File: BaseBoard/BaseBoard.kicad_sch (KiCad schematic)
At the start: 33 parts, among them J1 IMU, J13 Conn_01x02_Female, J14 Conn_01x03_Female, J2 Conn_01x04, J3 Raspberry_Pi_2_3, J4 USB_C_Receptacle_USB2.0, J5 Conn_02x04, SW1 SW_Push, SW2 SW_Push, U1 GD32VF103C8Tx, Y1 8Mhz

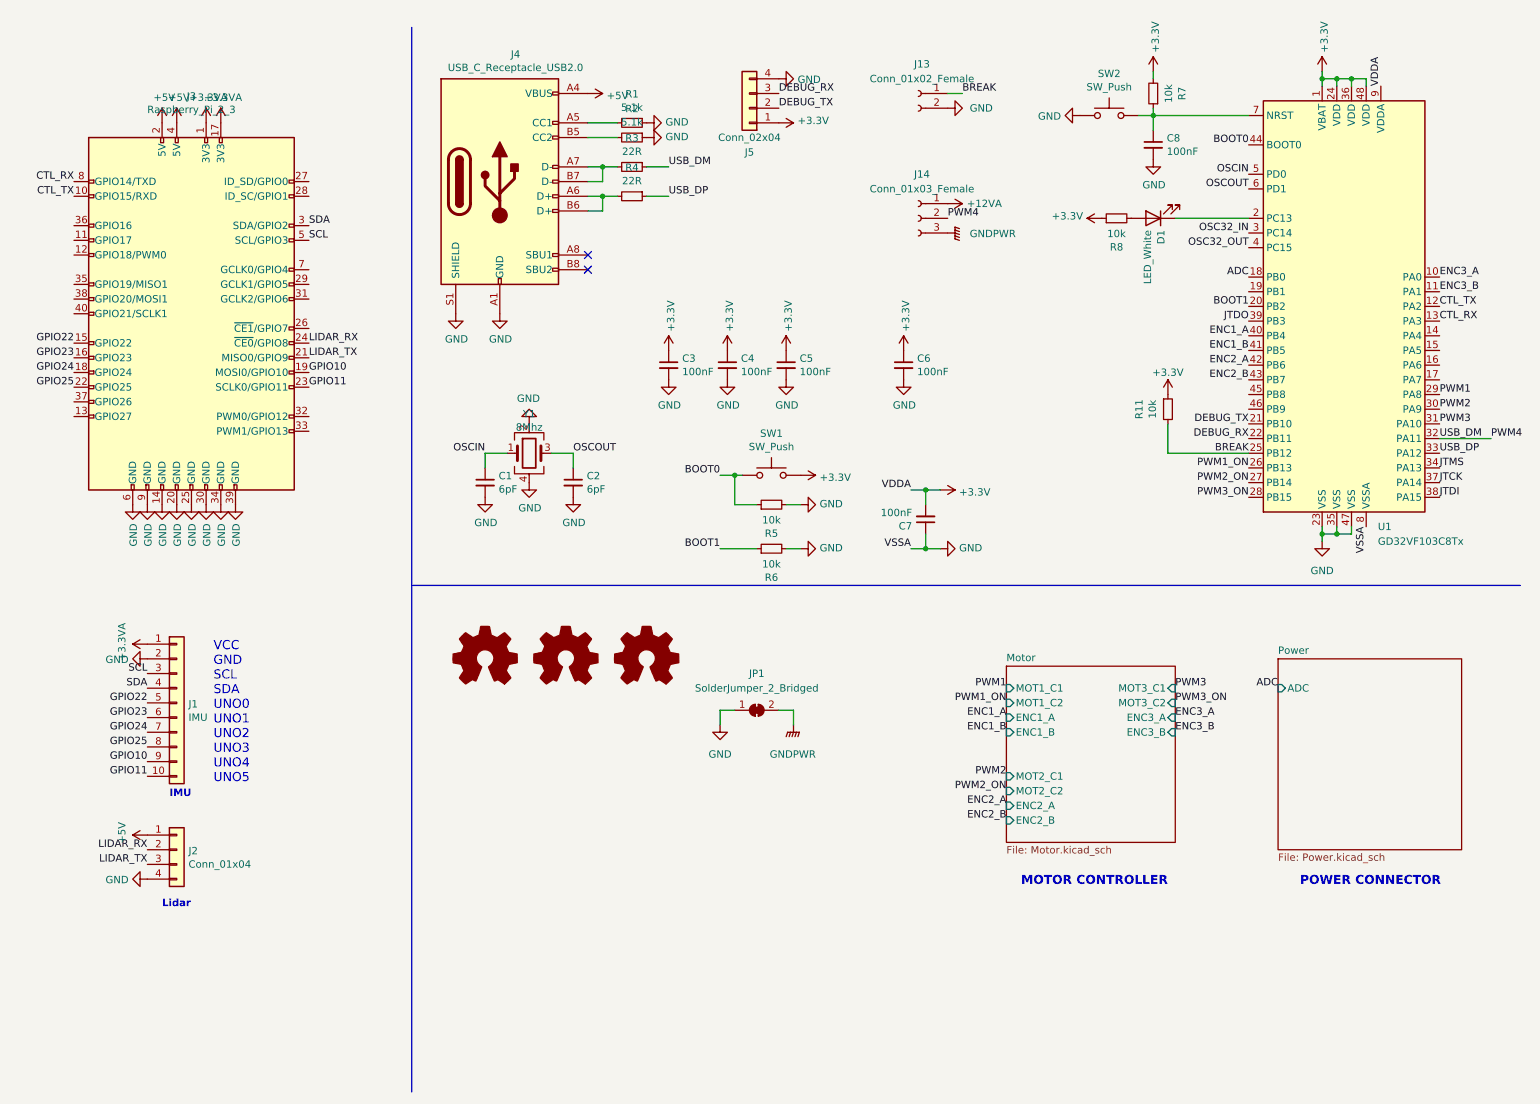
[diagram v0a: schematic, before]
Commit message: 更新V3线路板
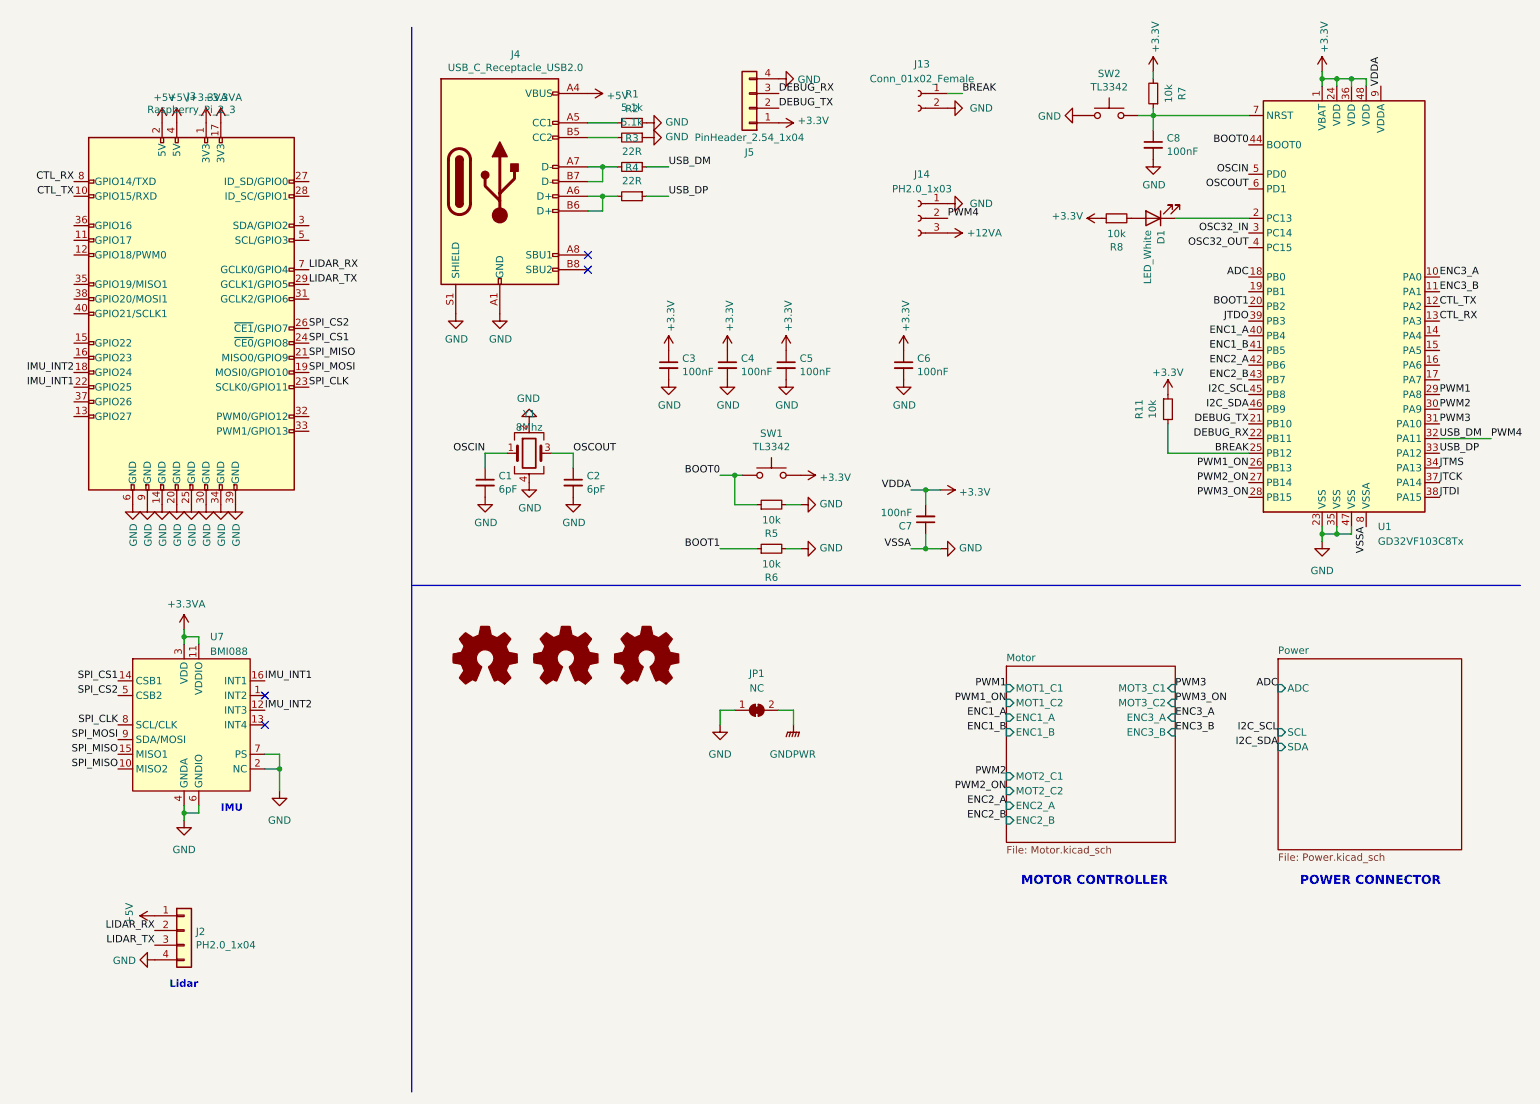
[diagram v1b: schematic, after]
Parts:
- removed J1: IMU, Connector_PinSocket_2.54mm:PinSocket_1x10_P2.54mm_Vertical, symbol Connector_Generic:Conn_01x10
- added U7: BMI088, Smallbot:Bochs_LGA16_2x7+2x1, symbol Smallbot:BMI088
- J14: value Conn_01x03_Female -> PH2.0_1x03
- J2: value Conn_01x04 -> PH2.0_1x04
- J5: value Conn_02x04 -> PinHeader_2.54_1x04
- JP1: value SolderJumper_2_Bridged -> NC
- SW1, SW2: value SW_Push -> TL3342; footprint User_Button_Switch:SW_SPST_EVQP7C-Single -> Button_Switch_SMD:SW_SPST_TL3342
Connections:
- net +12VA: now also J14.3 (Pin_3); no longer J14.1 (Pin_1)
- net +3.3VA: now also U7.11 (VDDIO), U7.3 (VDD)
- net GND: now also J14.1 (Pin_1), U7.2 (NC), U7.4 (GNDA), U7.6 (GNDIO), U7.7 (PS)
- net GNDPWR: no longer J14.3 (Pin_3)
- net LIDAR_RX: now also J3.7 (GCLK0/GPIO4); no longer J3.24 (~{CE0}/GPIO8)
- net LIDAR_TX: now also J3.29 (GCLK1/GPIO5); no longer J3.21 (MISO0/GPIO9)
- net SPI_CS2: now reaches J3.26 (~{CE1}/GPIO7)
- net SPI_CS2: now also U7.5 (CSB2)
- net I2C_SCL: now reaches U1.45 (PB8)
- net I2C_SDA: now reaches U1.46 (PB9)
- net GPIO10 renamed SPI_MOSI
- net SPI_MOSI: now also U7.9 (SDA/MOSI)
- net GPIO11 renamed SPI_CLK
- net SPI_CLK: now also U7.8 (SCL/CLK)
- net GPIO22: no longer names the net of J3.15 (GPIO22)
- net GPIO23: no longer names the net of J3.16 (GPIO23)
- net GPIO24 renamed IMU_INT2
- net IMU_INT2: now also U7.12 (INT3)
- net GPIO25 renamed IMU_INT1
- net IMU_INT1: now also U7.16 (INT1)
- net SCL: no longer names the net of J3.5 (SCL/GPIO3)
- net SDA: no longer names the net of J3.3 (SDA/GPIO2)
- new net SPI_CS1: J3.24 (~{CE0}/GPIO8), U7.14 (CSB1)
- new net SPI_MISO: J3.21 (MISO0/GPIO9), U7.10 (MISO2), U7.15 (MISO1)
- no-connect marks 2 -> 4
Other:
- sheet Power ports: added SCL, SDA; removed none
- note removed: "VCC GND SCL SDA UNO0 UNO1 UNO2 UNO3 UNO4 UNO5"
- moved on the sheet: J2
